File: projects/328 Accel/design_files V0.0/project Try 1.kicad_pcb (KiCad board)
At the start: 2 copper layers, 35 x 20.5 mm, 38 parts, among them CON1 ISP, J1 HL, J10 JST_PH, J2 CHG, J2 Molex_PicoBlade_53261-0271_02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, J3 BAT, J4 CONN, J44 CONN, J5 CONN, J55 CONN, J6 HL, J7 TL, J8 TL, J9 DSH, SW1 SW_SPDT, U1 ATMEGA328-MU, U2 LIS3DH

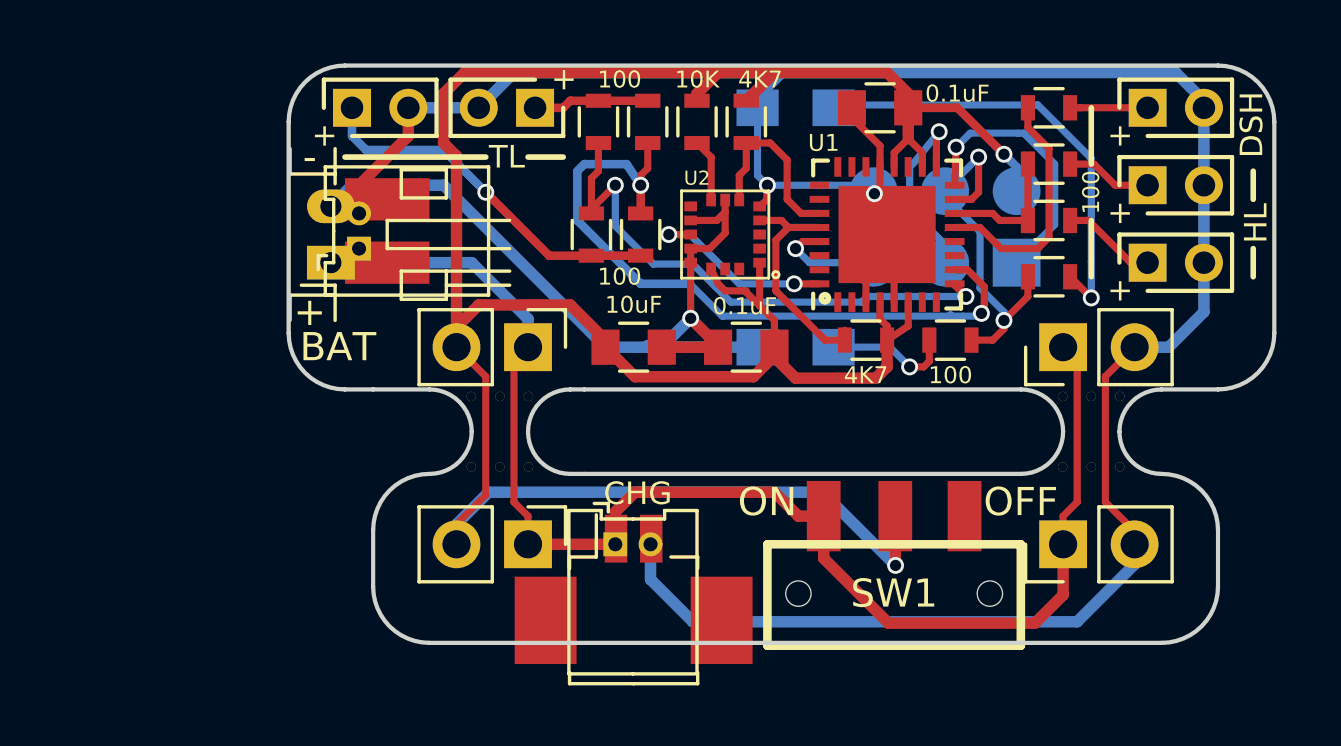
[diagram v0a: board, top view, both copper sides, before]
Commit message: Updates
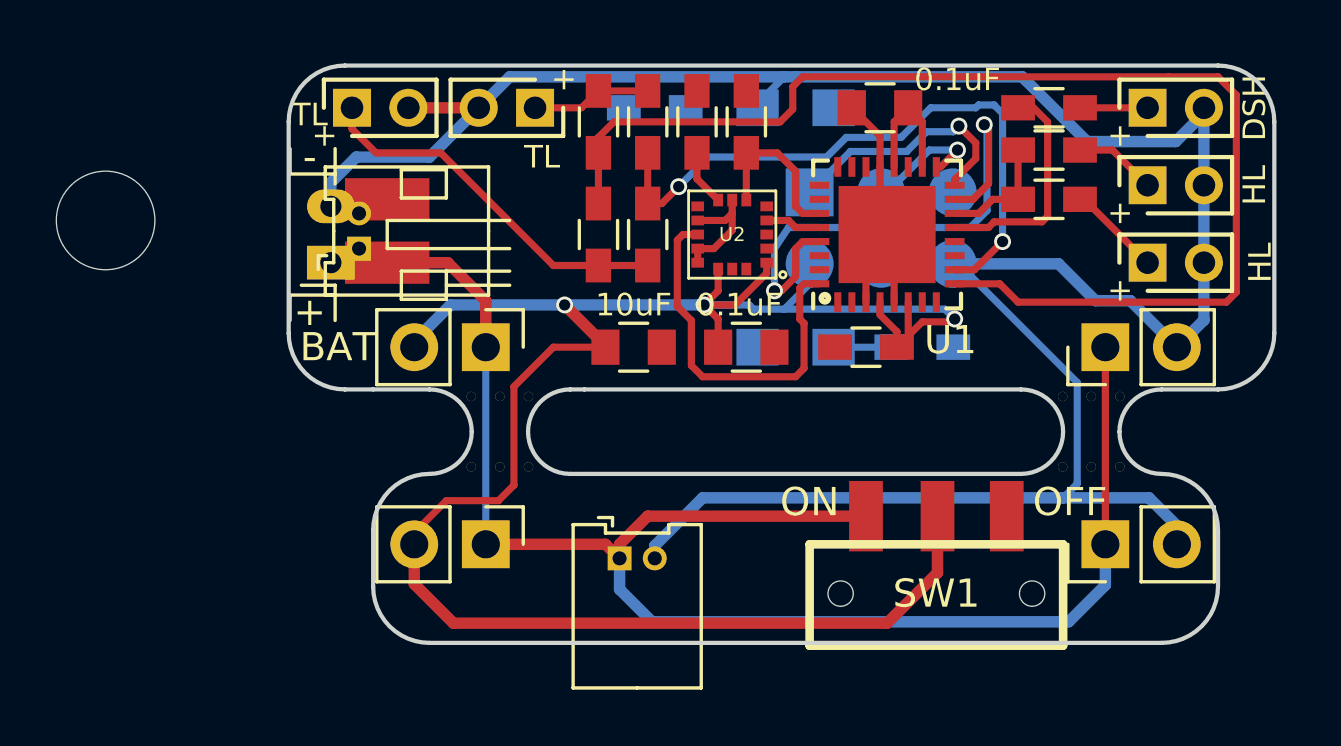
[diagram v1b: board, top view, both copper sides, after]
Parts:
- removed the J2 at (130.2, 162.8)
- added Drill: MountPad, Wire_Pads:SolderWirePad_single_2mmDrill, F.Cu at (111.5, 150.0)
- R1, R10, R2, R3, R4, R5, R6, R7, R8, R9: footprint footprints:R_0603 -> footprints:R_0603_HandSoldering
- R11, R12: footprint footprints:R_0603 -> footprints:R_0603_HandSoldering; moved to B.Cu
- moved R12 15.2 mm to (131.0, 146.0), turned to 180 degrees
- moved CON1 7.76 mm to (136.5, 149.0), turned to 270 degrees
- moved J4 1.50 mm to (125.0, 161.5)
- moved J44 1.50 mm to (125.0, 154.5)
- moved J5 1.50 mm to (147.0, 161.5)
- moved J55 1.50 mm to (147.0, 154.5)
- moved SW1 1.50 mm to (141.0, 160.5)
- moved R11 1.03 mm to (140.5, 154.5)
- moved R7 0.75 mm to (145.0, 149.2)
- moved J2 0.52 mm to (129.8, 162.0)
- moved R6 0.50 mm to (145.0, 147.5)
- moved R3 0.25 mm to (138.5, 154.5)
- moved R4 0.25 mm to (129.0, 150.5)
- moved R8 0.25 mm to (130.8, 150.5)
- moved U2 0.25 mm to (133.8, 150.5)
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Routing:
- net /D5: track 19.7 -> 44.0 mm, vias 2 -> 0
- net GND: track 128.8 -> 109.2 mm, vias 3 -> 0
- net Net-(D5-Pad2): track 16.0 -> 0.25 mm, vias 1 -> 0
- net VCC: track 94.5 -> 79.1 mm, vias 2 -> 3
- net /~RESET: track 3.93 -> 11.8 mm
- net /D2: track 6.85 -> 13.4 mm, vias 2 -> 0
- net Net-(J10-Pad1): track 50.3 -> 56.7 mm
- net /SCL: track 8.19 -> 1.98 mm
- net /D6: track 25.3 -> 22.6 mm
- net /SCK: track 6.85 -> 4.33 mm
- net Net-(D4-Pad2): track 4.52 -> 2.45 mm, vias 1 -> 0
- net /MOSI: track 12.9 -> 12.0 mm, vias 2 -> 1
- net /SDA: track 6.58 -> 5.90 mm
- net /D9: track 8.74 -> 8.07 mm
- net /MISO: track 9.57 -> 8.93 mm
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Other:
- board text removed: "328 Accel"
